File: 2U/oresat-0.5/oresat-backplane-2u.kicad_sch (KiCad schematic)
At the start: 59 parts, among them J1 m55-6001642

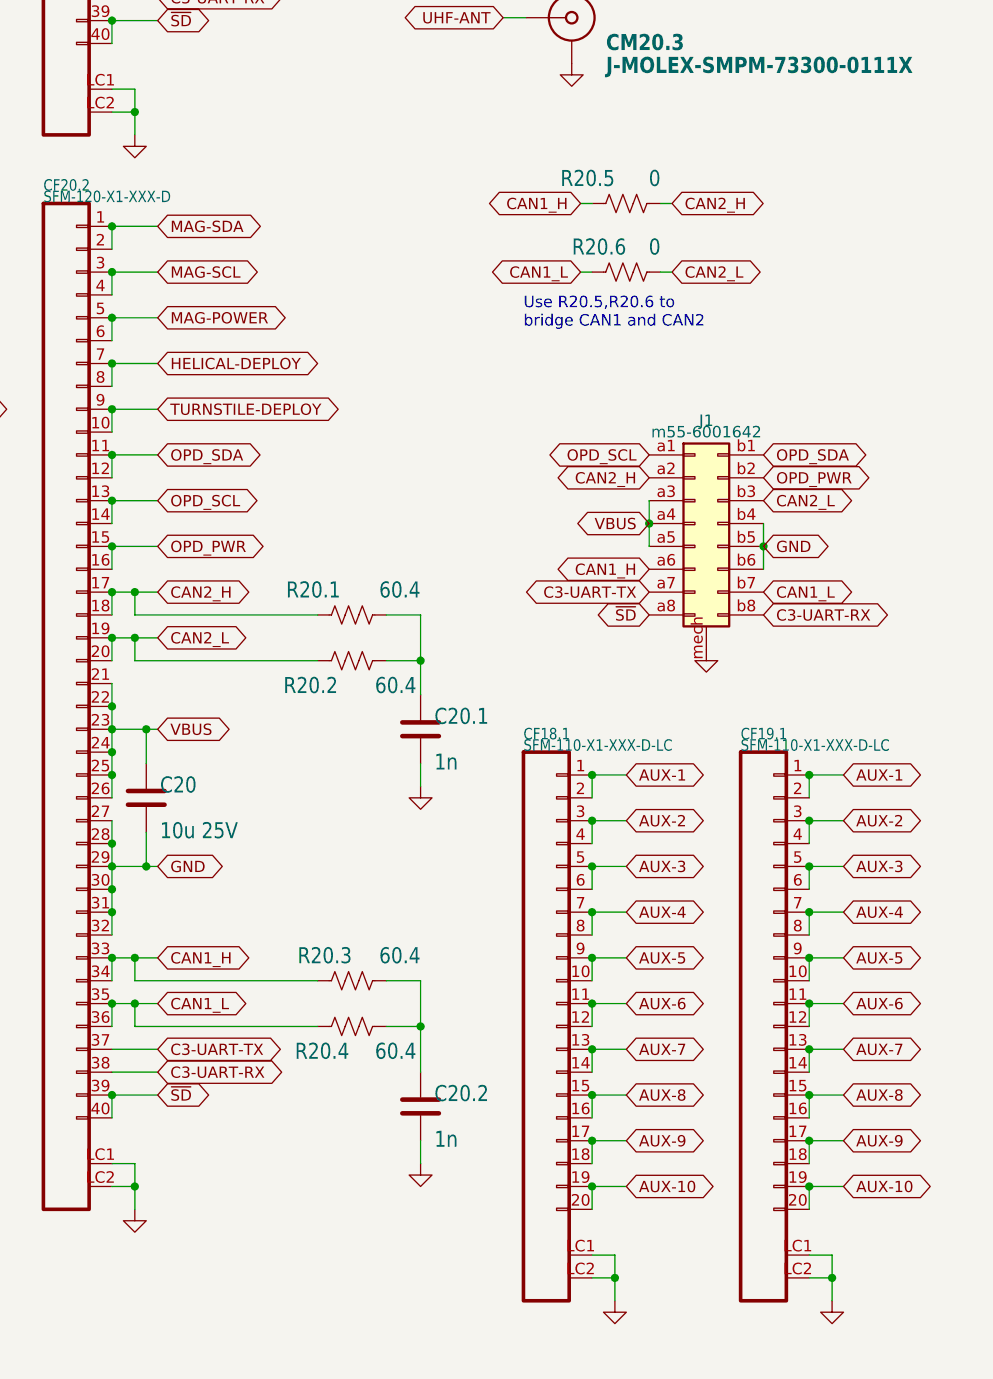
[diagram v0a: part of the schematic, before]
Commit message: Ready for fab I think
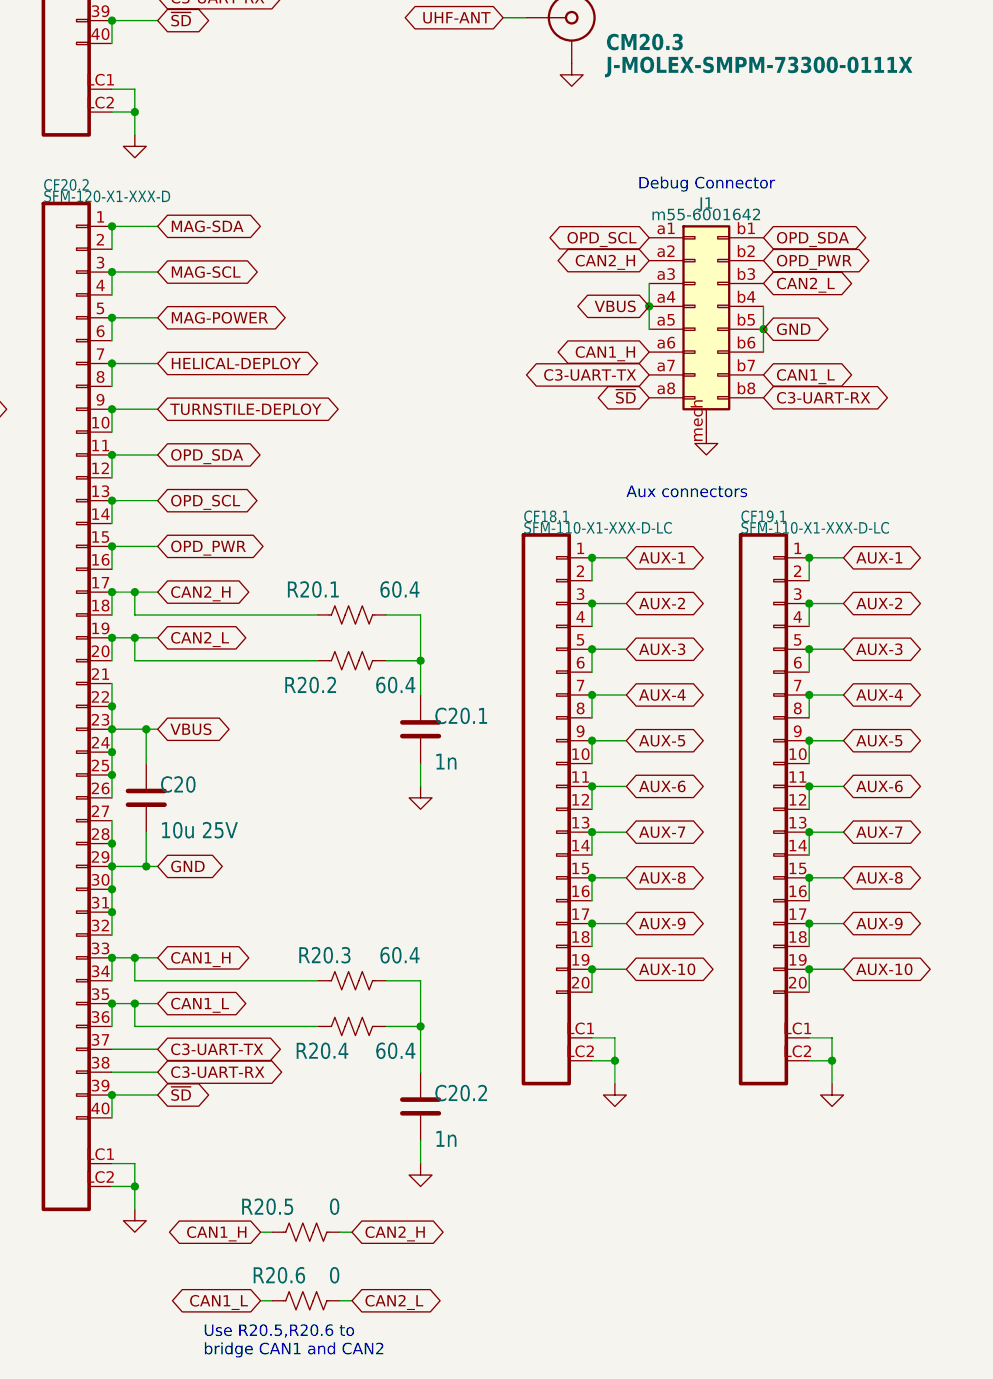
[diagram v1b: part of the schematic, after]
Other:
- note added: "Aux connectors"
- note added: "Debug Connector"
- moved on the sheet: CF18.1, CF19.1, J1, R20.5, R20.6

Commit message: Fixed backplane connector library names
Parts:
- CF1.2, CF12.2, CF13.2, CF14.2, CF15.2, CF16.2, CF17.2, CF18.2, CF19.2, CF2.2, CF20.2, CF3.2, CF4.2, CF5.2, CF6.2, CF7.2, CF8.2: symbol oresat-connectors:J-SAMTEC-TFM-120-01-L-D-RA -> oresat-connectors:J-SAMTEC-SFM-120-X1-XXX-D
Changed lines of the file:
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@@
     )
   )
-  (symbol (lib_id "oresat-connectors:J-SAMTEC-TFM-120-01-L-D-RA") (at 283.21 186.69 0) (unit 1)
+  (symbol (lib_id "oresat-connectors:J-SAMTEC-SFM-120-X1-XXX-D") (at 283.21 186.69 0) (unit 1)
     (in_bom yes) (on_board yes)
     (property "Reference" "CF19.2" (id 0) (at 280.67 134.62 0)
@@
     (pin "2")
   )
-  (symbol (lib_id "oresat-connectors:J-SAMTEC-TFM-120-01-L-D-RA") (at 172.72 186.69 0) (unit 1)
+  (symbol (lib_id "oresat-connectors:J-SAMTEC-SFM-120-X1-XXX-D") (at 172.72 186.69 0) (unit 1)
     (in_bom yes) (on_board yes)
     (property "Reference" "CF16.2" (id 0) (at 170.18 134.62 0)
@@
     (pin "2")
   )
-  (symbol (lib_id "oresat-connectors:J-SAMTEC-TFM-120-01-L-D-RA") (at 320.04 67.31 0) (unit 1)
+  (symbol (lib_id "oresat-connectors:J-SAMTEC-SFM-120-X1-XXX-D") (at 320.04 67.31 0) (unit 1)
     (in_bom yes) (on_board yes)
     (property "Reference" "CF8.2" (id 0) (at 317.5 15.24 0)
@@
     (pin "1")
   )
-  (symbol (lib_id "oresat-connectors:J-SAMTEC-TFM-120-01-L-D-RA") (at 25.4 186.69 0) (unit 1)
+  (symbol (lib_id "oresat-connectors:J-SAMTEC-SFM-120-X1-XXX-D") (at 25.4 186.69 0) (unit 1)
     (in_bom yes) (on_board yes)
     (property "Reference" "CF12.2" (id 0) (at 22.86 134.62 0)
@@
     (pin "1")
   )
-  (symbol (lib_id "oresat-connectors:J-SAMTEC-TFM-120-01-L-D-RA") (at 209.55 67.31 0) (unit 1)
+  (symbol (lib_id "oresat-connectors:J-SAMTEC-SFM-120-X1-XXX-D") (at 209.55 67.31 0) (unit 1)
     (in_bom yes) (on_board yes)
     (property "Reference" "CF5.2" (id 0) (at 207.01 15.24 0)
@@
     (pin "1")
   )
-  (symbol (lib_id "oresat-connectors:J-SAMTEC-TFM-120-01-L-D-RA") (at 135.89 67.31 0) (unit 1)
+  (symbol (lib_id "oresat-connectors:J-SAMTEC-SFM-120-X1-XXX-D") (at 135.89 67.31 0) (unit 1)
     (in_bom yes) (on_board yes)
     (property "Reference" "CF3.2" (id 0) (at 133.35 15.24 0)
@@
     (pin "mech")
   )
-  (symbol (lib_id "oresat-connectors:J-SAMTEC-TFM-120-01-L-D-RA") (at 25.4 68.58 0) (unit 1)
+  (symbol (lib_id "oresat-connectors:J-SAMTEC-SFM-120-X1-XXX-D") (at 25.4 68.58 0) (unit 1)
     (in_bom yes) (on_board yes)
     (property "Reference" "CF1.2" (id 0) (at 22.86 16.51 0)
@@
     (pin "LC2")
   )
-  (symbol (lib_id "oresat-connectors:J-SAMTEC-TFM-120-01-L-D-RA") (at 99.06 67.31 0) (unit 1)
+  (symbol (lib_id "oresat-connectors:J-SAMTEC-SFM-120-X1-XXX-D") (at 99.06 67.31 0) (unit 1)
     (in_bom yes) (on_board yes)
     (property "Reference" "CF2.2" (id 0) (at 96.52 15.24 0)
@@
     (pin "1")
   )
-  (symbol (lib_id "oresat-connectors:J-SAMTEC-TFM-120-01-L-D-RA") (at 99.06 186.69 0) (unit 1)
+  (symbol (lib_id "oresat-connectors:J-SAMTEC-SFM-120-X1-XXX-D") (at 99.06 186.69 0) (unit 1)
     (in_bom yes) (on_board yes)
     (property "Reference" "CF14.2" (id 0) (at 96.52 134.62 0)
@@
     (pin "LC2")
   )
-  (symbol (lib_id "oresat-connectors:J-SAMTEC-TFM-120-01-L-D-RA") (at 283.21 67.31 0) (unit 1)
+  (symbol (lib_id "oresat-connectors:J-SAMTEC-SFM-120-X1-XXX-D") (at 283.21 67.31 0) (unit 1)
     (in_bom yes) (on_board yes)
     (property "Reference" "CF7.2" (id 0) (at 280.67 15.24 0)
@@
     (pin "1")
   )
-  (symbol (lib_id "oresat-connectors:J-SAMTEC-TFM-120-01-L-D-RA") (at 246.38 186.69 0) (unit 1)
+  (symbol (lib_id "oresat-connectors:J-SAMTEC-SFM-120-X1-XXX-D") (at 246.38 186.69 0) (unit 1)
     (in_bom yes) (on_board yes)
     (property "Reference" "CF18.2" (id 0) (at 243.84 134.62 0)
@@
     (pin "2")
   )
-  (symbol (lib_id "oresat-connectors:J-SAMTEC-TFM-120-01-L-D-RA") (at 172.72 67.31 0) (unit 1)
+  (symbol (lib_id "oresat-connectors:J-SAMTEC-SFM-120-X1-XXX-D") (at 172.72 67.31 0) (unit 1)
     (in_bom yes) (on_board yes)
     (property "Reference" "CF4.2" (id 0) (at 170.18 15.24 0)
@@
     (pin "1")
   )
-  (symbol (lib_id "oresat-connectors:J-SAMTEC-TFM-120-01-L-D-RA") (at 209.55 186.69 0) (unit 1)
+  (symbol (lib_id "oresat-connectors:J-SAMTEC-SFM-120-X1-XXX-D") (at 209.55 186.69 0) (unit 1)
     (in_bom yes) (on_board yes)
     (property "Reference" "CF17.2" (id 0) (at 207.01 134.62 0)
@@
     (pin "1")
   )
-  (symbol (lib_id "oresat-connectors:J-SAMTEC-TFM-120-01-L-D-RA") (at 62.23 186.69 0) (unit 1)
+  (symbol (lib_id "oresat-connectors:J-SAMTEC-SFM-120-X1-XXX-D") (at 62.23 186.69 0) (unit 1)
     (in_bom yes) (on_board yes)
     (property "Reference" "CF13.2" (id 0) (at 59.69 134.62 0)
@@
     (pin "LC2")
   )
-  (symbol (lib_id "oresat-connectors:J-SAMTEC-TFM-120-01-L-D-RA") (at 320.04 186.69 0) (unit 1)
+  (symbol (lib_id "oresat-connectors:J-SAMTEC-SFM-120-X1-XXX-D") (at 320.04 186.69 0) (unit 1)
     (in_bom yes) (on_board yes)
     (property "Reference" "CF20.2" (id 0) (at 317.5 134.62 0)
@@
     (pin "2")
   )
-  (symbol (lib_id "oresat-connectors:J-SAMTEC-TFM-120-01-L-D-RA") (at 135.89 186.69 0) (unit 1)
+  (symbol (lib_id "oresat-connectors:J-SAMTEC-SFM-120-X1-XXX-D") (at 135.89 186.69 0) (unit 1)
     (in_bom yes) (on_board yes)
     (property "Reference" "CF15.2" (id 0) (at 133.35 134.62 0)
@@
     (pin "2")
   )
-  (symbol (lib_id "oresat-connectors:J-SAMTEC-TFM-120-01-L-D-RA") (at 246.38 67.31 0) (unit 1)
+  (symbol (lib_id "oresat-connectors:J-SAMTEC-SFM-120-X1-XXX-D") (at 246.38 67.31 0) (unit 1)
     (in_bom yes) (on_board yes)
     (property "Reference" "CF6.2" (id 0) (at 243.84 15.24 0)
